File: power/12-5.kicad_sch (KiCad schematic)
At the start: 9 parts, among them U4 RPM5.0-6.0, U5 HO8-NP

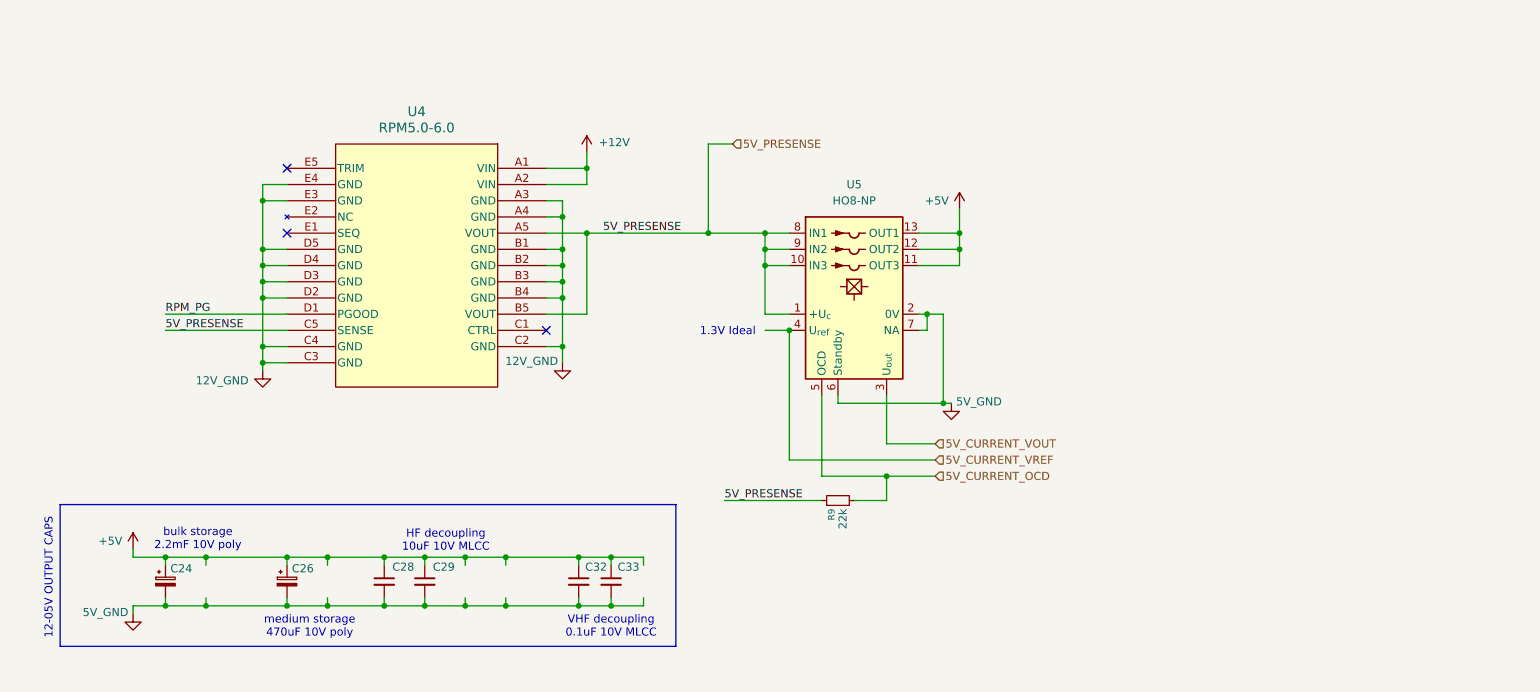
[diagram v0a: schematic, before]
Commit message: work
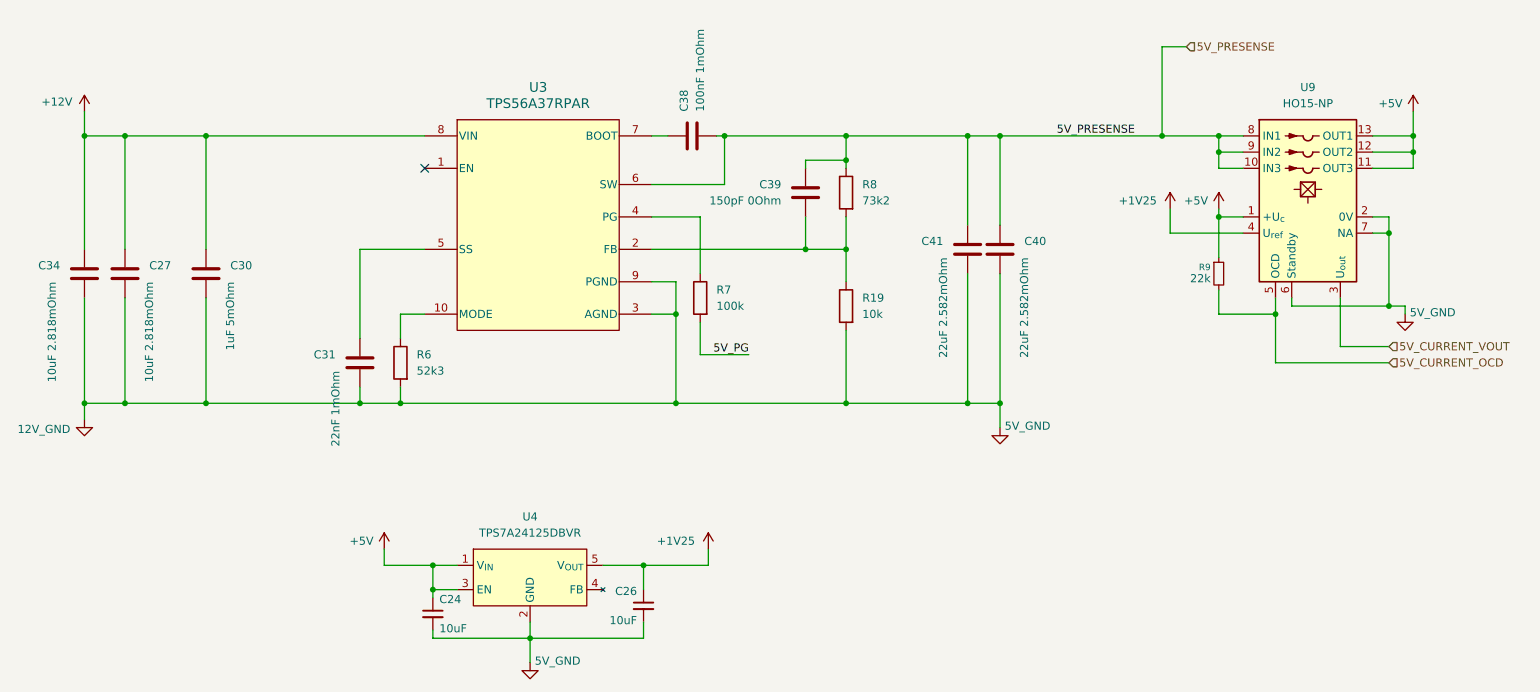
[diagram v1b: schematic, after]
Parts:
- removed C24, C26: C_Polarized_Small, Capacitor_THT:CP_Radial_D10.0mm_P5.00mm, symbol Device:C_Polarized_Small
- removed C28, C29, C32, C33: C_Small, Capacitor_SMD:C_0603_1608Metric, symbol Device:C_Small
- removed U4: RPM5.0-6.0, power_symbols:RPM5.0-6.0, symbol power_symbols:RPM5.0-6.0
- removed U5: HO8-NP, Sensor_Current:LEM_HO8-NP, symbol Sensor_Current:HO8-NP
- added C24, C26: 10uF, Capacitor_SMD:C_0603_1608Metric, symbol Device:C_Small
- added C27, C34: 10uF 2.818mOhm, symbol Device:C
- added C30: 1uF 5mOhm, symbol Device:C
- added C31: 22nF 1mOhm, symbol Device:C
- added C38: 100nF 1mOhm, symbol Device:C
- added C39: 150pF 0Ohm, symbol Device:C
- added C40, C41: 22uF 2.582mOhm, symbol Device:C
- added R19: 10k, symbol Device:R
- added R6: 52k3, symbol Device:R
- added R7: 100k, symbol Device:R
- added R8: 73k2, symbol Device:R
- added U3: TPS56A37RPAR, custom:TPS56A37RPAR, symbol custom:TPS56A37RPAR
- added U4: TPS7A24125DBVR, Package_TO_SOT_SMD:SOT-23-5, symbol custom:TPS7A24125DBVR
- added U9: HO15-NP, Sensor_Current:LEM_HO8-NP, symbol Sensor_Current:HO15-NP
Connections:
- net +12V: now also C27.1, C30.1, C34.1, U3.8 (VIN)
- net +5V: now also R9.1, C24.1, U4.1 (V_{IN}), U4.3 (EN), U9.1 (+U_{c}), U9.11 (OUT3), U9.12 (OUT2), U9.13 (OUT1)
- net 12V_GND: now also C24.2, C26.2, C27.2, C30.2, C31.2, C34.2, C40.2, C41.2, R19.2, R6.2, U3.3 (AGND), U3.9 (PGND), U4.2 (GND), U9.2 (0V), U9.6 (Standby), U9.7 (NA)
- net 5V_CURRENT_OCD: now also U9.5 (OCD)
- net 5V_CURRENT_VOUT: now also U9.3 (U_{out})
- net 5V_PRESENSE: now also C38.2, C39.1, C40.1, C41.1, R8.1, U3.6 (SW), U9.10 (IN3), U9.8 (IN1), U9.9 (IN2); no longer R9.1
- new net: C31.1, U3.5 (SS)
- new net: R6.1, U3.10 (MODE)
- new net: C39.2, R19.1, R8.2, U3.2 (FB)
- new net: R7.1, U3.4 (PG)
- new net: C38.1, U3.7 (BOOT)
- new net +1V25: C26.1, U4.5 (V_{OUT}), U9.4 (U_{ref})
- new net 5V_PG: R7.2
- no-connect marks 3 -> 1
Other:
- note removed: "1.3V Ideal"
- note removed: "12-05V OUTPUT CAPS"
- note removed: "HF decoupling 10uF 10V MLCC"
- note removed: "VHF decoupling 0.1uF 10V MLCC"
- note removed: "bulk storage 2.2mF 10V poly"
- note removed: "medium storage 470uF 10V poly"
- moved on the sheet: R9
